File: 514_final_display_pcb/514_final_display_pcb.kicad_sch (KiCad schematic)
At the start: 12 parts, among them SW1 SW_Push, SW2 SW_Push, SW3 SW_Push, U1 MOUDLE-SEEEDUINO-XIAO-ESP32C3

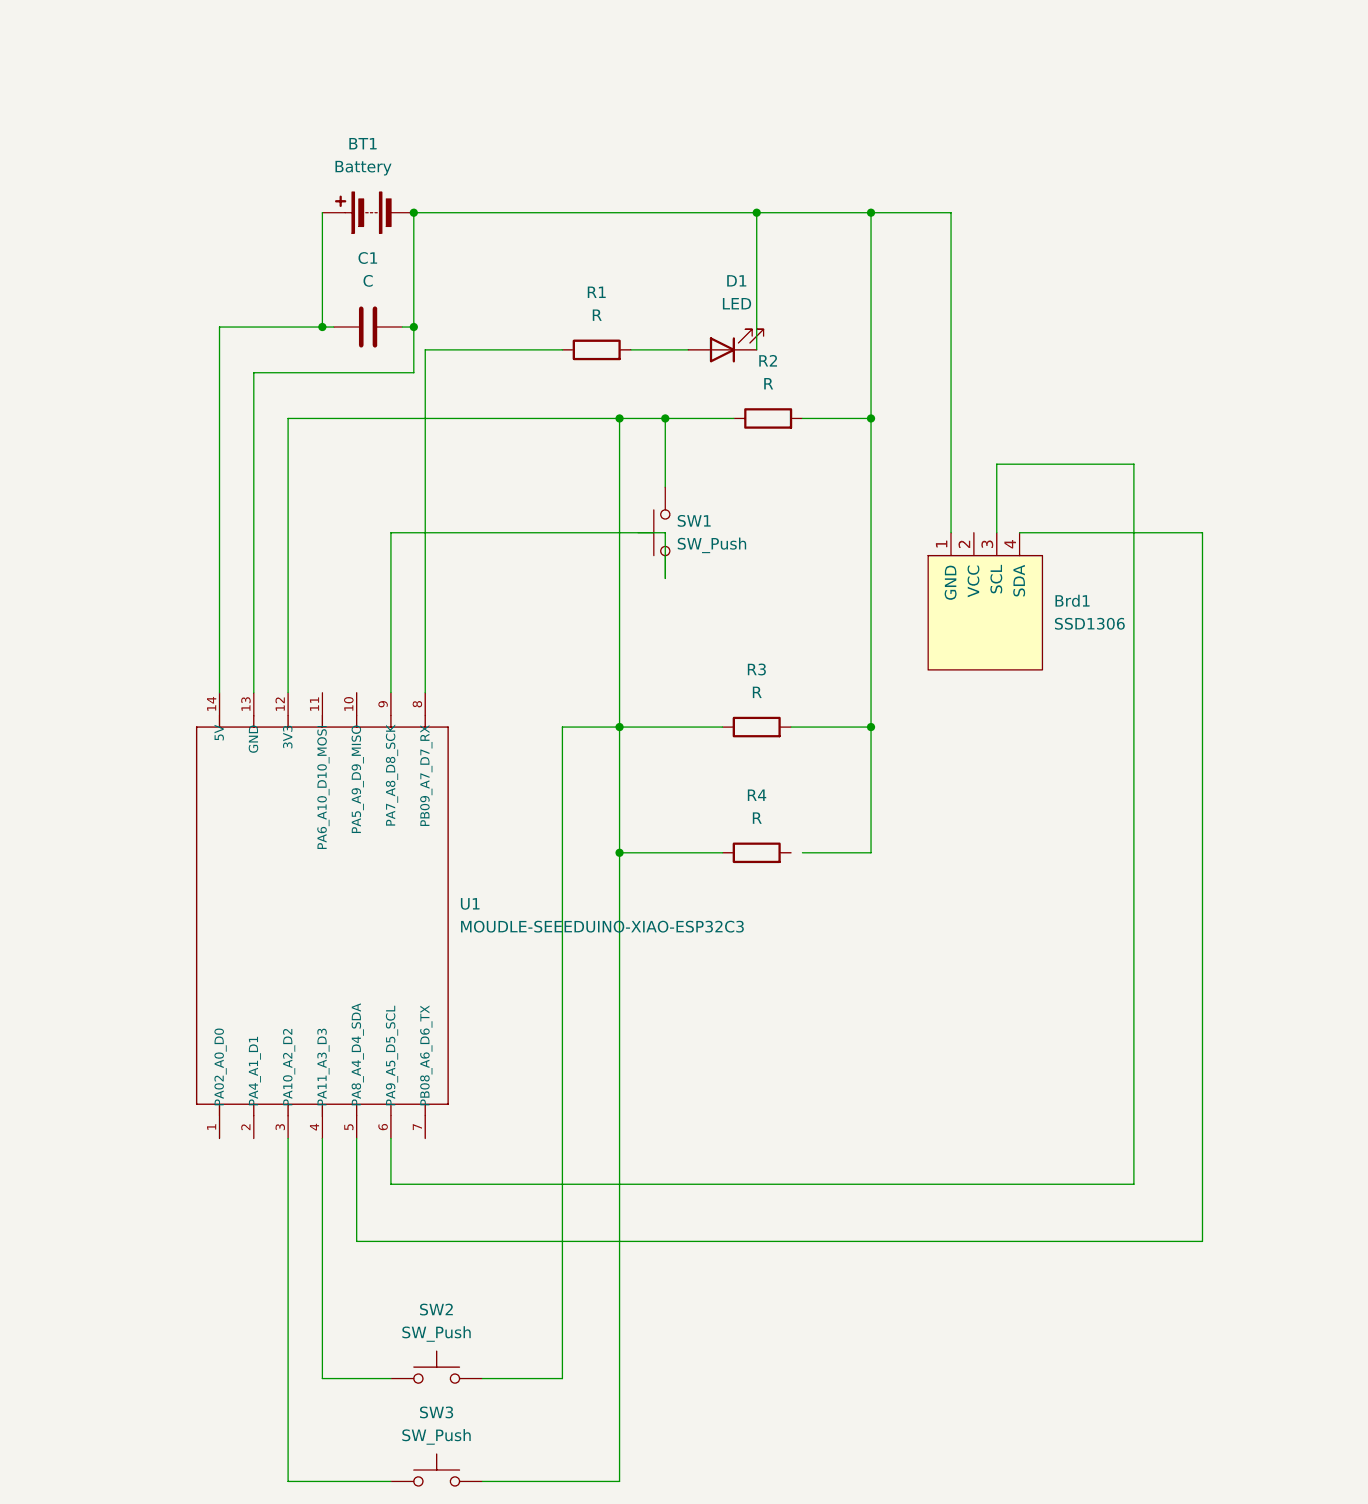
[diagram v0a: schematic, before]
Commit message: second device
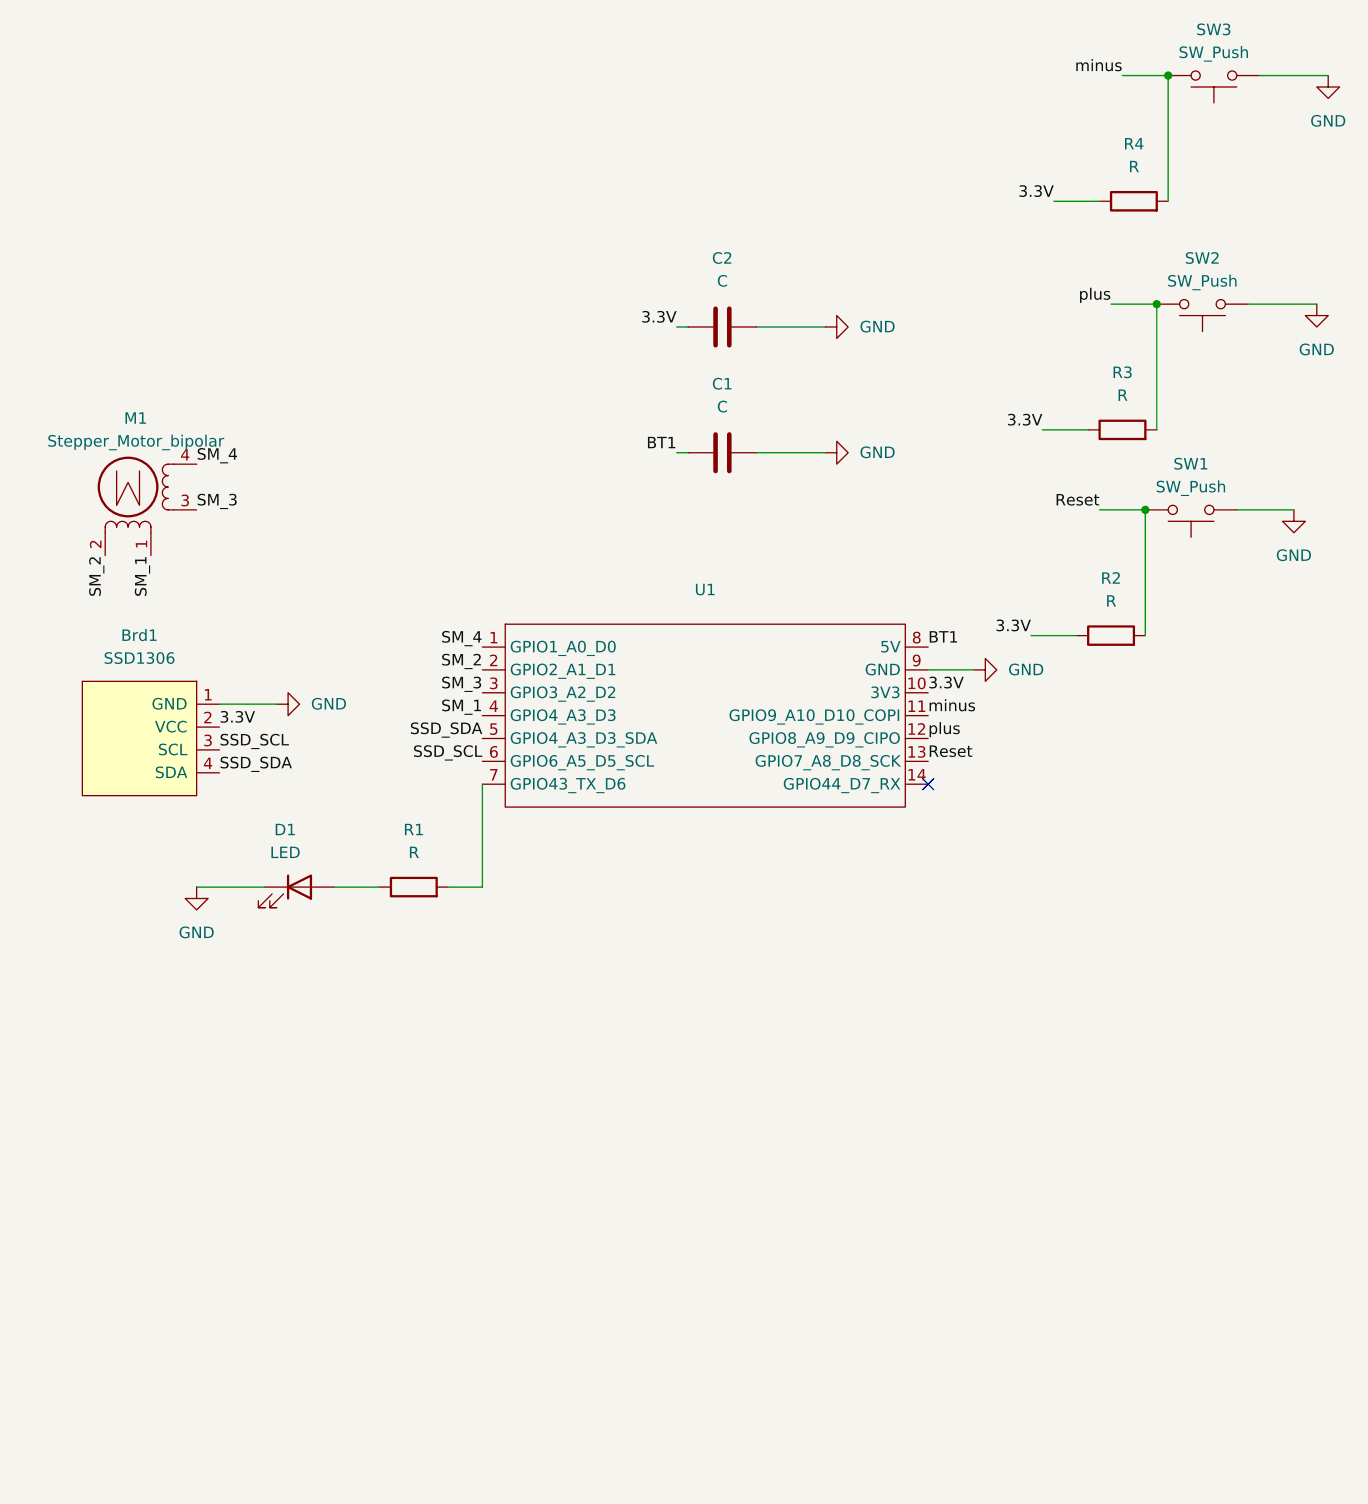
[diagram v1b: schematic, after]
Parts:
- removed BT1: Battery, symbol Device:Battery
- removed U1: MOUDLE-SEEEDUINO-XIAO-ESP32C3, MOUDLE14P-SMD-2.54-21X17.8MM, symbol MOUDLE-SEEEDUINO-XIAO-ESP32C3:MOUDLE-SEEEDUINO-XIAO-ESP32C3
- added C2: C, Capacitor_SMD:C_0805_2012Metric_Pad1.18x1.45mm_HandSolder, symbol Device:C
- added M1: Stepper_Motor_bipolar, Stepper Motor:x27_stepper_two_holes, symbol Motor:Stepper_Motor_bipolar
- added U1: ~, ESP32c3:XIAO_ESP32_SENSE, symbol ESP32C3:XIAO_ESP32_SENSE
- Brd1: footprint (none) -> SSD1306:128x64OLED
- C1: footprint (none) -> Capacitor_SMD:C_0805_2012Metric_Pad1.18x1.45mm_HandSolder
- D1: footprint (none) -> LED_THT:LED_D5.0mm
- R1, R2, R3, R4: footprint (none) -> Resistor_SMD:R_0805_2012Metric_Pad1.20x1.40mm_HandSolder
- SW1, SW2, SW3: footprint (none) -> Button_Switch_THT:SW_PUSH_6mm
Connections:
- net BT1: now reaches C1.1
- net BT1: now also U1.8 (5V)
- net GND: now reaches Brd1.1 (GND), C1.2, D1.1 (K)
- net GND: now also SW1.1, SW2.1, SW3.1, C2.2, U1.9 (GND); no longer R2.2, R3.2
- net 3.3V: now reaches R2.1, R3.1, R4.1
- net 3.3V: now also Brd1.2 (VCC), C2.1, U1.10 (3V3); no longer SW1.2, SW2.2, SW3.2
- net at R1.1: now also D1.2 (A)
- net at R1.2: now also U1.7 (GPIO43_TX_D6); no longer D1.2 (A)
- net minus: now reaches R4.2
- net minus: now also SW3.2, U1.11 (GPIO9_A10_D10_COPI)
- net SSD_SDA: now reaches Brd1.4 (SDA)
- net SSD_SDA: now also U1.5 (GPIO4_A3_D3_SDA)
- net SSD_SCL: now reaches Brd1.3 (SCL)
- net SSD_SCL: now also U1.6 (GPIO6_A5_D5_SCL)
- new net Reset: R2.2, SW1.2, U1.13 (GPIO7_A8_D8_SCK)
- new net SM_1: M1.1, U1.4 (GPIO4_A3_D3)
- new net SM_2: M1.2 (-), U1.2 (GPIO2_A1_D1)
- new net SM_3: M1.3, U1.3 (GPIO3_A2_D2)
- new net SM_4: M1.4, U1.1 (GPIO1_A0_D0)
- new net plus: R3.2, SW2.2, U1.12 (GPIO8_A9_D9_CIPO)
- no-connect marks 0 -> 1
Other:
- moved on the sheet: Brd1, C1, D1, R1, R2, SW1
